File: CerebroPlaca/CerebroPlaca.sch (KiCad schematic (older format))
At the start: 39 parts, among them J1 Connector_Generic_Conn_01x02, J2 USB_C_Receptacle_USB2.0, J3 Conn_01x08_Male, Q1 AO3407A, SW1 Switch_SW_SPDT, U1 AP2112K-3.3, U2 E73-2G4M08S1C-52840, U3 MCP73831-2-OT, Y1 Crystal

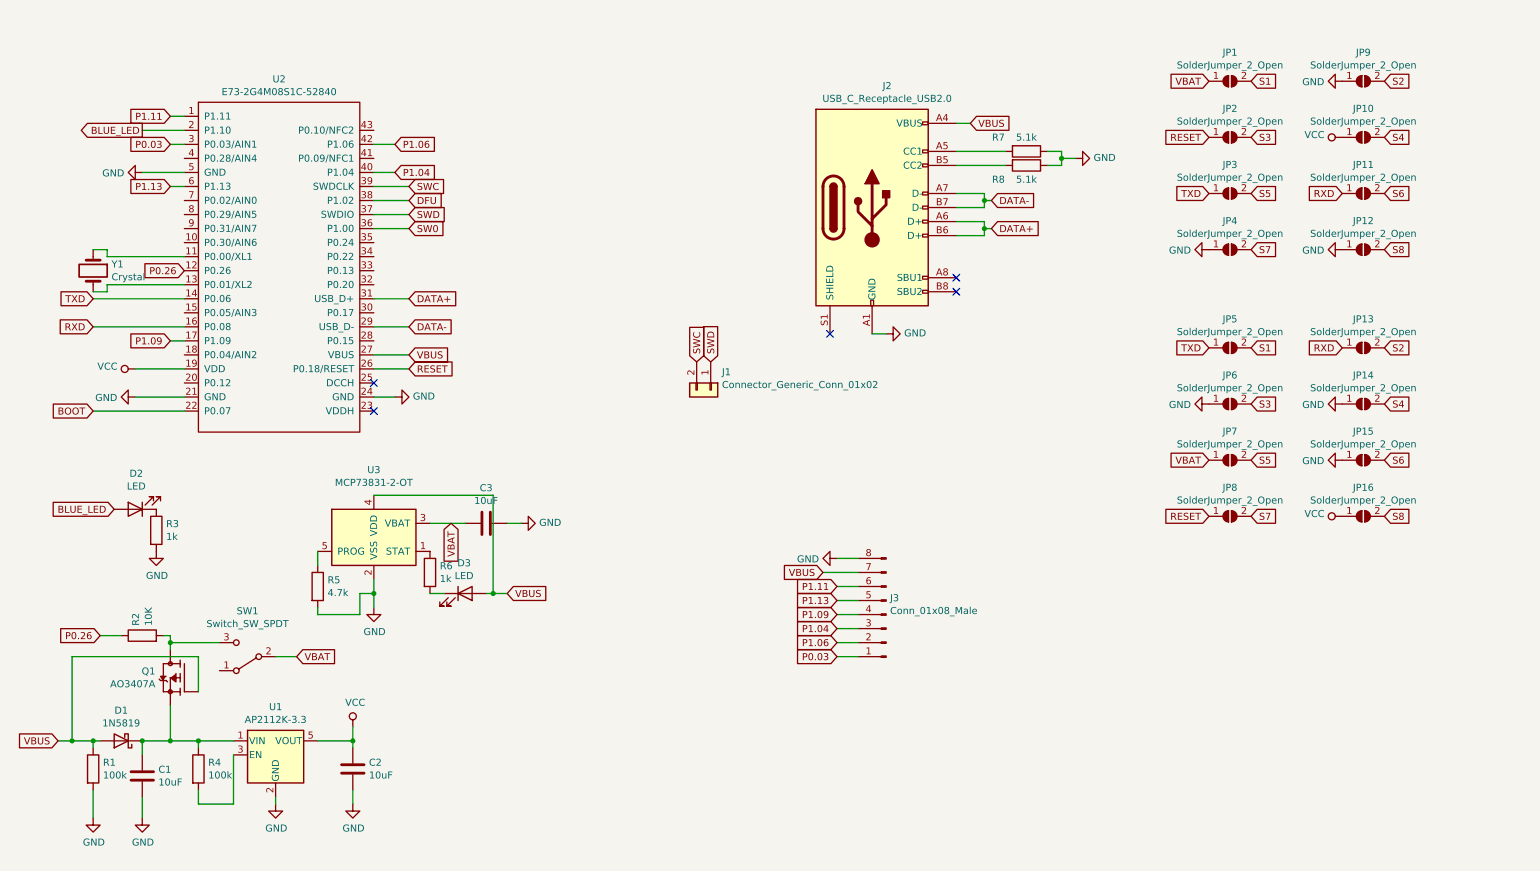
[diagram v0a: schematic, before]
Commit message: ajustes en placaCerebro
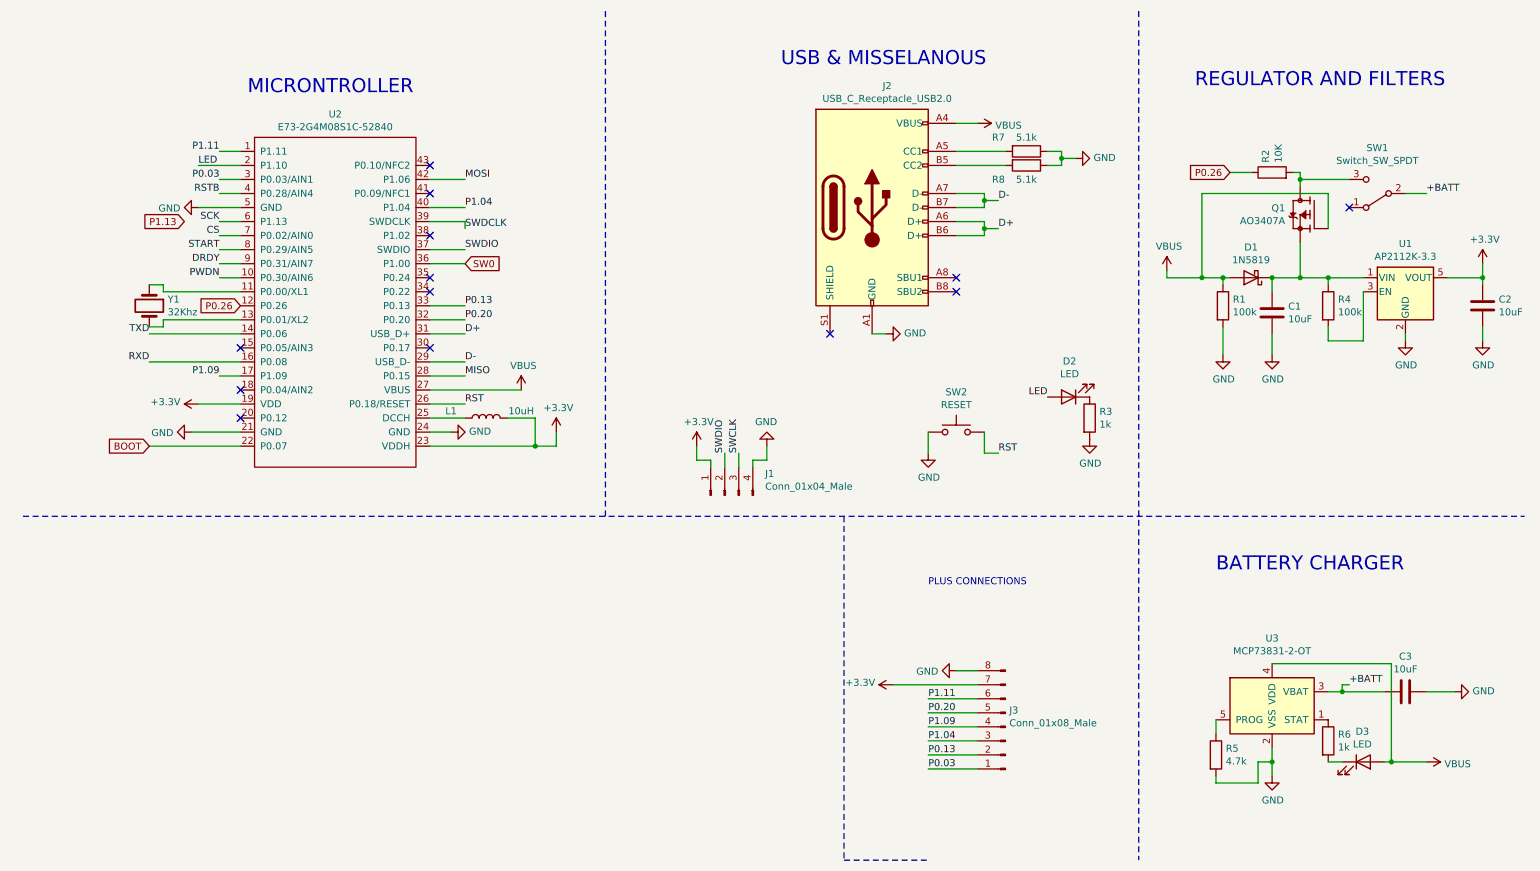
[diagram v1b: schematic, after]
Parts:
- removed J1: Connector_Generic_Conn_01x02, nrfmicro:connector_swd, symbol cerebro-cache:Connector_Generic_Conn_01x02
- removed JP1, JP10, JP11, JP12, JP13, JP14, JP15, JP16, JP2, JP3, JP4, JP5, JP6, JP7, JP8, JP9: SolderJumper_2_Open, nrfmicro:jumper, symbol Jumper:SolderJumper_2_Open
- added J1: Conn_01x04_Male, Connector_PinHeader_1.00mm:PinHeader_1x04_P1.00mm_Vertical, symbol Connector:Conn_01x04_Male
- added L1: 10uH, Inductor_SMD:L_7.3x7.3_H3.5, symbol Device:L
- added SW2: RESET, Button_Switch_SMD:SW_SPST_TL3342, symbol Switch:SW_MEC_5G
- Y1: value Crystal -> 32Khz
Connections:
- net VCC is gone; now on net +3V3: C2.1, U1.5 (VOUT), U2.19 (VDD)
- net GND: now also J1.4 (Pin_4), SW2.1 (A), SW2.2 (A)
- net P1.13: no longer J3.5 (Pin_5), U2.6 (P1.13)
- net VBUS: no longer J3.7 (Pin_7)
- net PWDN: now reaches U2.10 (P0.30/AIN6)
- net +3V3: now reaches U2.23 (VDDH)
- net +3V3: now also J3.7 (Pin_7), J1.1 (Pin_1), L1.2
- net at U2.25 (DCCH): now also L1.1
- net MISO: now reaches U2.28 (P0.15)
- net P0.20: now reaches U2.32 (P0.20)
- net P0.20: now also J3.5 (Pin_5)
- net P0.13: now reaches U2.33 (P0.13)
- net P0.13: now also J3.2 (Pin_2)
- net RSTB: now reaches U2.4 (P0.28/AIN4)
- net CS: now reaches U2.7 (P0.02/AIN0)
- net START: now reaches U2.8 (P0.29/AIN5)
- net DRDY: now reaches U2.9 (P0.31/AIN7)
- net BLUE_LED renamed LED
- net DATA+ renamed D+
- net DATA- renamed D-
- net DFU: no longer names the net of U2.38 (P1.02)
- net P1.06 renamed MOSI
- net MOSI: no longer J3.2 (Pin_2)
- net RESET renamed RST
- net RST: now also SW2.3 (B), SW2.4 (B)
- net SWC renamed SWDCLK
- net SWD renamed SWDIO
- net SWDIO: now also J1.2 (Pin_2)
- net VBAT renamed +BATT
- new net SCK: U2.6 (P1.13)
- new net SWCLK: J1.3 (Pin_3)
- no-connect marks 5 -> 13
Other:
- note added: "BATTERY CHARGER"
- note added: "MICRONTROLLER"
- note added: "PLUS CONNECTIONS"
- note added: "REGULATOR AND FILTERS"
- note added: "USB & MISSELANOUS"
- moved on the sheet: C1, C2, C3, D1, D2, D3, J3, Q1, R1, R2, R3, R4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
